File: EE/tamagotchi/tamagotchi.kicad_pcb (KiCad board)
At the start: 4 copper layers, 34.8 x 38.8 mm, 46 parts, among them J1 Conn_01x02_Male, J3 Conn_01x07, J7 TAG_CONNECT, J8 Conn_01x02_Male, P1 USB_C_Plug_USB2.0, Q1 Q_NMOS_GSD, Q2 Q_NMOS_GSD, Q4 Q_NMOS_GSD, Q5 Q_PMOS_GSD, SW2 TL1260BQRBLK, U2 STM32G031G8Ux

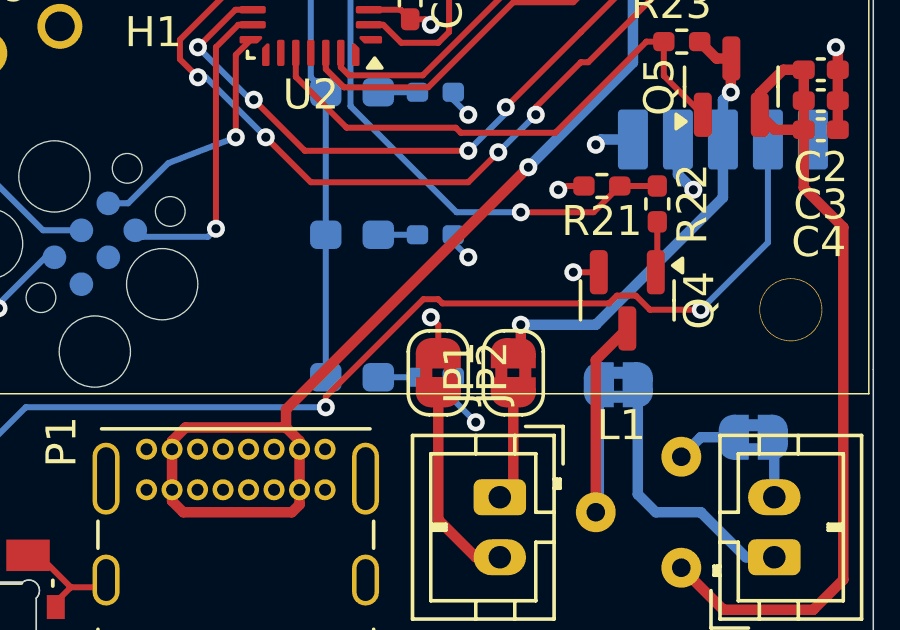
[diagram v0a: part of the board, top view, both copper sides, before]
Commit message: Silkscreen Fix
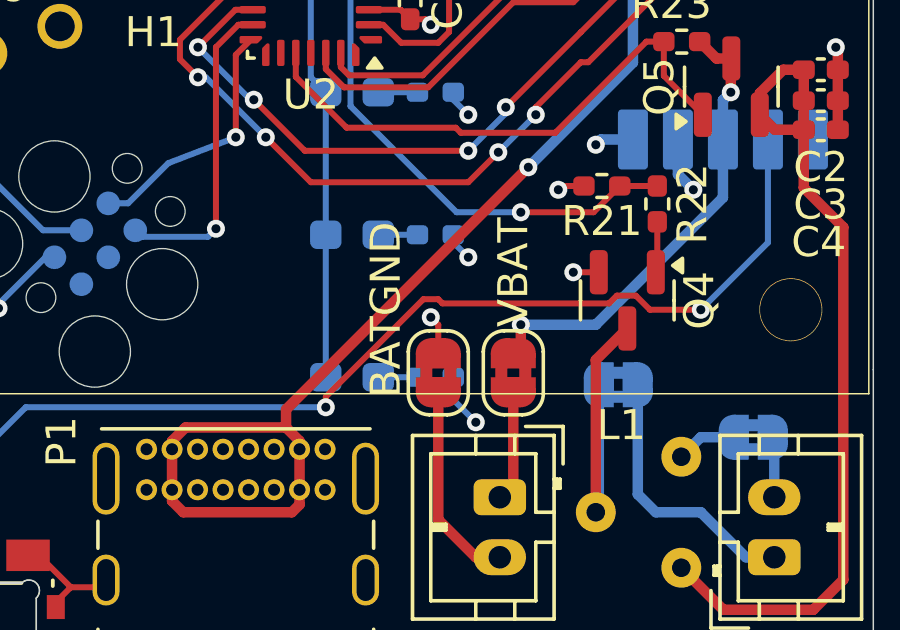
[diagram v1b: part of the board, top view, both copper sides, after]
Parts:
- renumbered JP2 to BATGND, JP4 to UT+, JP3 to UT-, JP1 to VBAT
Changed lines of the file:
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@@
 		(descr "SMD Solder Jumper, 1x1.5mm, rounded Pads, 0.3mm gap, bridged with 2 copper strips")
 		(tags "net tie solder jumper bridged")
-		(property "Reference" "JP1"
-			(at 0 -1.8 90)
+		(property "Reference" "VBAT"
+			(at 3.350001 0 90)
 			(layer "F.SilkS")
 			(effects
@@
 		(descr "SMD Solder Jumper, 1x1.5mm, rounded Pads, 0.3mm gap, bridged with 2 copper strips")
 		(tags "net tie solder jumper bridged")
-		(property "Reference" "JP2"
-			(at 0 -1.8 90)
+		(property "Reference" "BATGND"
+			(at -2.100001 1.75 90)
 			(layer "F.SilkS")
 			(effects
@@
 		(at 160.2375 86.175 -90)
 		(property "Reference" "U1"
-			(at 0 1 90)
+			(at 1.575 0.7375 90)
 			(unlocked yes)
 			(layer "B.SilkS")
@@
 		(descr "SMD Solder Jumper, 1x1.5mm, rounded Pads, 0.3mm gap, bridged with 2 copper strips")
 		(tags "net tie solder jumper bridged")
-		(property "Reference" "JP4"
+		(property "Reference" "UT+"
 			(at 0 1.8 0)
 			(layer "B.SilkS")
@@
 		(descr "SMD Solder Jumper, 1x1.5mm, rounded Pads, 0.3mm gap, bridged with 2 copper strips")
 		(tags "net tie solder jumper bridged")
-		(property "Reference" "JP3"
+		(property "Reference" "UT-"
 			(at 0 1.8 0)
 			(layer "B.SilkS")
